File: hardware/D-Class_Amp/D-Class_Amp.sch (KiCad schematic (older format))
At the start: 31 parts, among them J101 P_IN, J102 AudioJack2, U101 NCP1117-12_TO252, U102 MCP1799T-5002H_TT

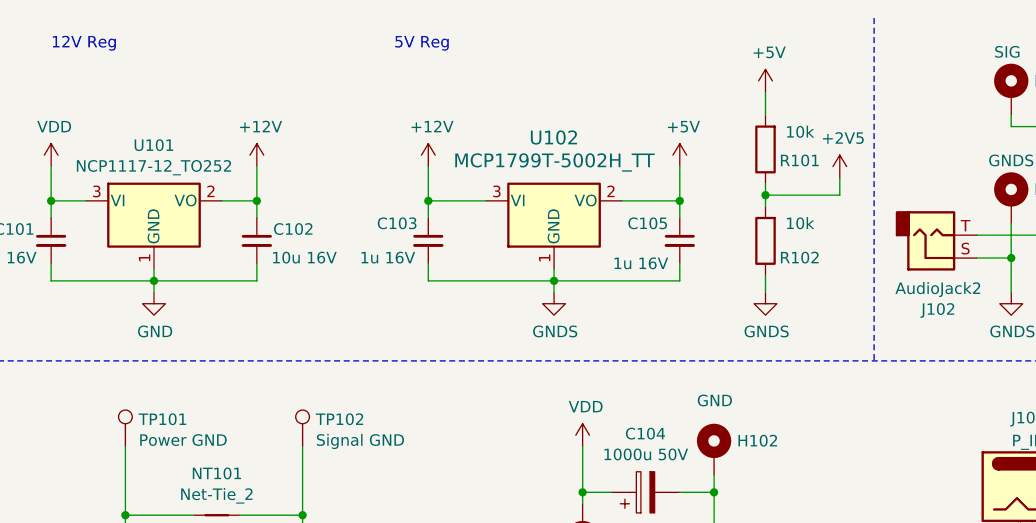
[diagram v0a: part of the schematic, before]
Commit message: update design
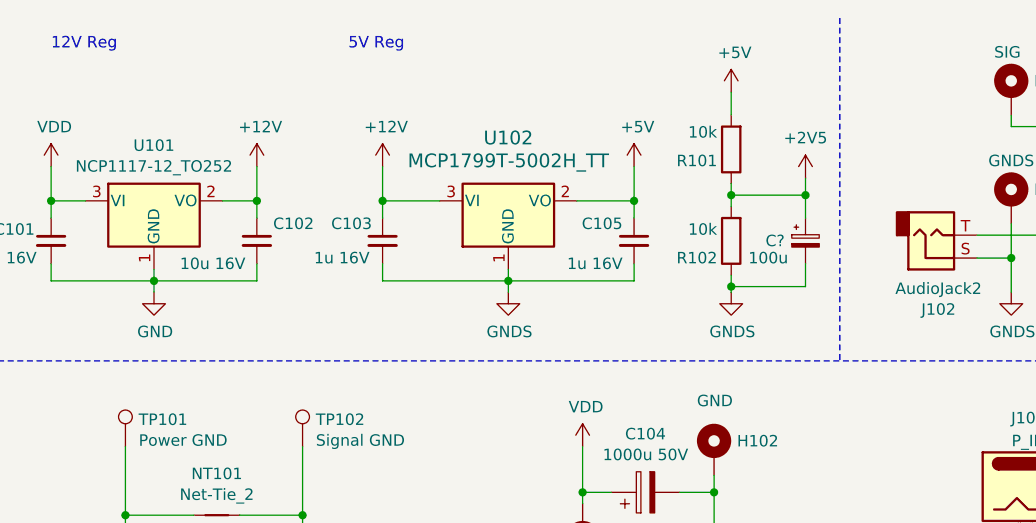
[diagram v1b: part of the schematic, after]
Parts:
- added C?: 100u, Capacitor_SMD:CP_Elec_4x5.4, symbol Device:CP_Small
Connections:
- net +2V5: now also C?.1
- net GNDS: now also C?.2
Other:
- moved on the sheet: C103, C105, R101, R102, U102
